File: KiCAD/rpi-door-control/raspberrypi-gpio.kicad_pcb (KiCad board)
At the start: 2 copper layers, 85 x 56 mm, 9 parts, among them P1 CONN_13X2

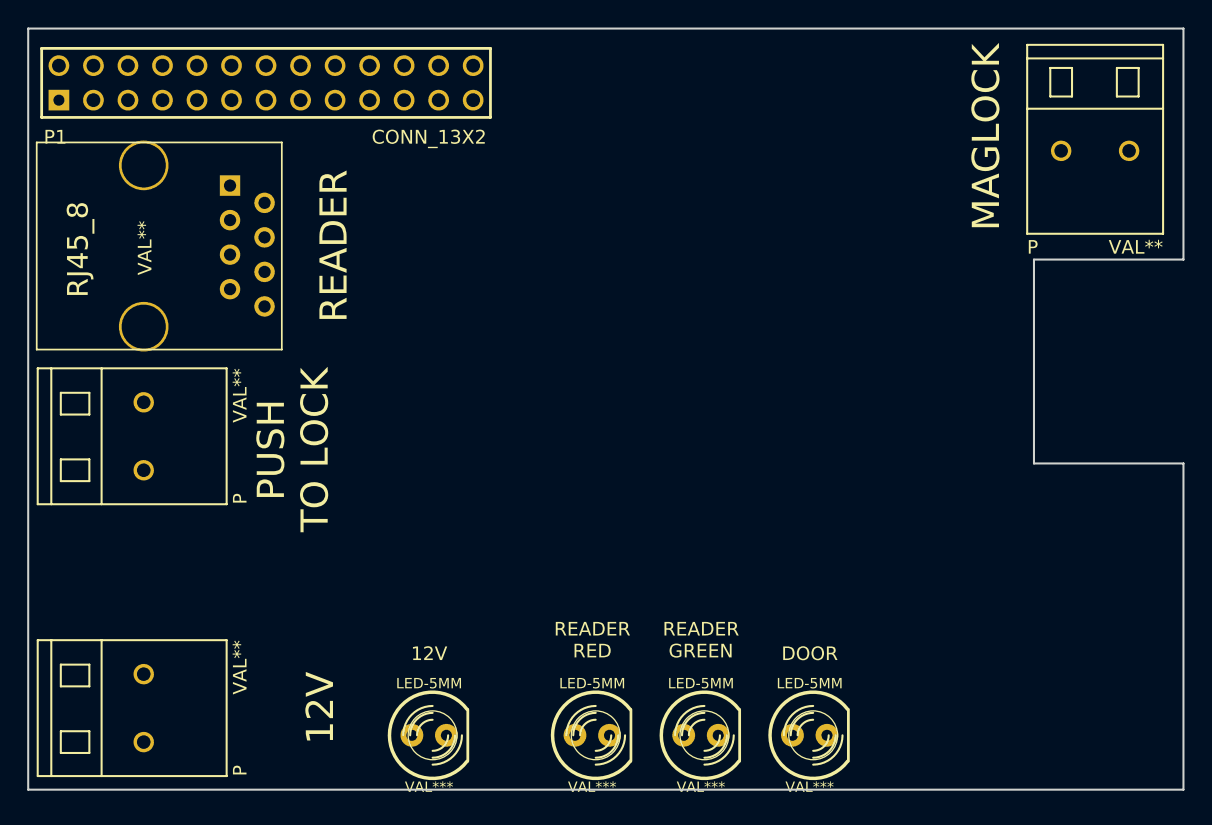
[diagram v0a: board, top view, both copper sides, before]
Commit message: components placed - who knows if the layout is any good or not
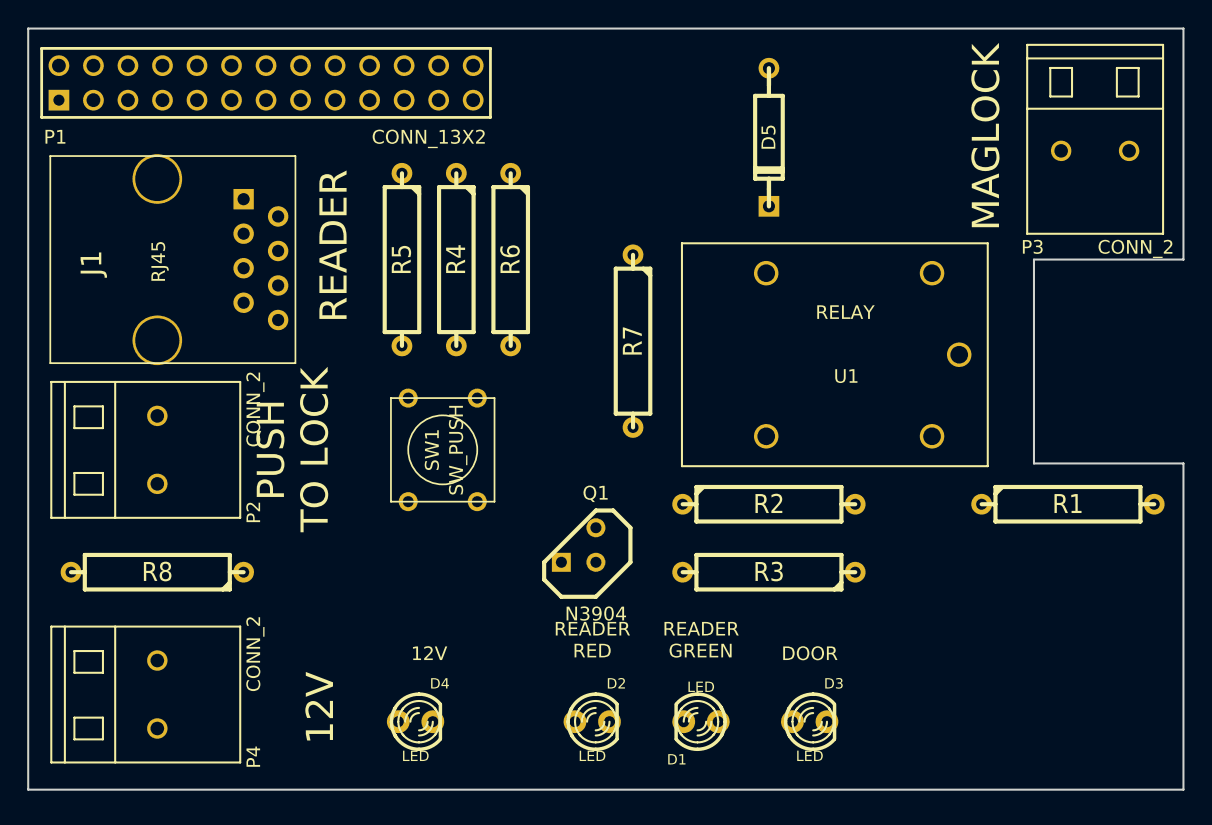
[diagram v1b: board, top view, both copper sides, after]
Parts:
- removed LED-5MM (x4): VAL***, LED-5MM
- removed P (x3): VAL**, 2Pole_Terminal_block
- removed RJ45_8: VAL**, RJ45_8
- added D1: LED, LED-3MM, F.Cu at (193.0, 176.0)
- added D2: LED, LED-3MM, F.Cu at (185.0, 176.0)
- added D3: LED, LED-3MM, F.Cu at (201.0, 176.0)
- added D4: LED, LED-3MM, F.Cu at (172.0, 176.0)
- added D5: 1N4007, DO-41, F.Cu at (198.0, 133.0)
- added J1: RJ45, RJ45_8, F.Cu at (153.0, 142.0)
- added P2: CONN_2, C2_KF103, F.Cu at (153.0, 156.0)
- added P3: CONN_2, C2_KF103, F.Cu at (222.0, 134.0)
- added P4: CONN_2, C2_KF103, F.Cu at (153.0, 174.0)
- added Q1: N3904, TO92, F.Cu at (184.0, 163.0)
- added R1: 10K, R5, F.Cu at (220.0, 160.0)
- added R2: 1.8K, R5, F.Cu at (198.0, 160.0)
- added R3: 3.3K, R5, F.Cu at (198.0, 165.0)
- added R4: 330, R5, F.Cu at (175.0, 142.0)
- added R5: 330, R5, F.Cu at (171.0, 142.0)
- added R6: 330, R5, F.Cu at (179.0, 142.0)
- added R7: 1K, R5, F.Cu at (188.0, 148.0)
- added R8: 2K, R5, F.Cu at (153.0, 165.0)
- added SW1: SW_PUSH, SW_PUSH_SMALL, F.Cu at (174.0, 156.0)
- added U1: RELAY, RELAY_AZ942, F.Cu at (210.0, 149.0)
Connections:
- P1 pad 10: (no net) -> /RXD
- P1 pad 11: (no net) -> /GPIO17
- P1 pad 13: (no net) -> /BELL
- P1 pad 16: (no net) -> /GPIO23
- P1 pad 18: (no net) -> /GPIO24
- P1 pad 22: (no net) -> /GPIO25
